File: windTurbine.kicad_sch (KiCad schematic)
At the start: 12 parts, among them M1 Motor_Servo, M2 LP-MSPM0G3507

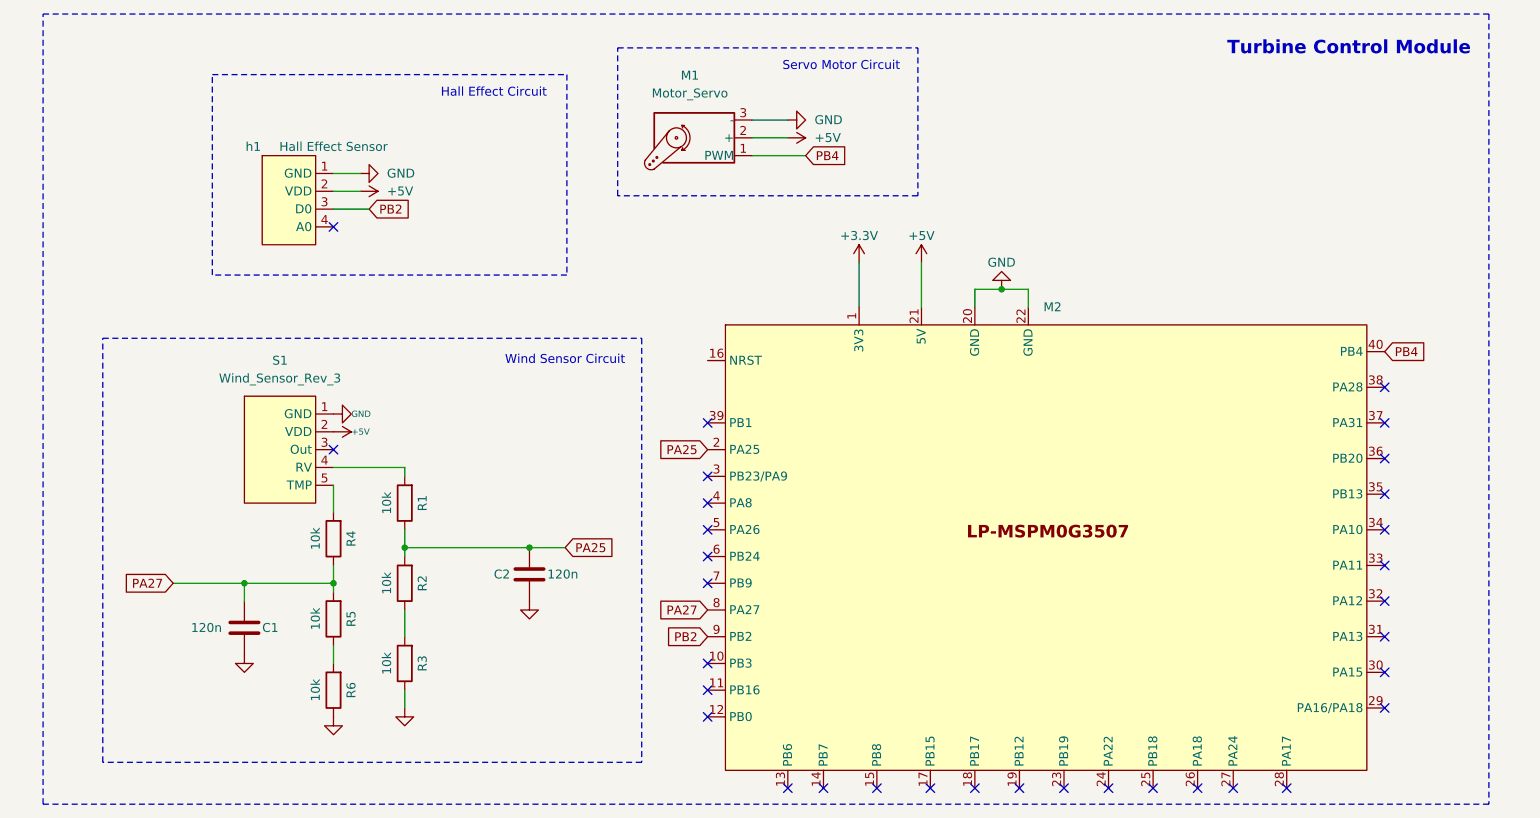
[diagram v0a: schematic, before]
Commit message: Load MCU
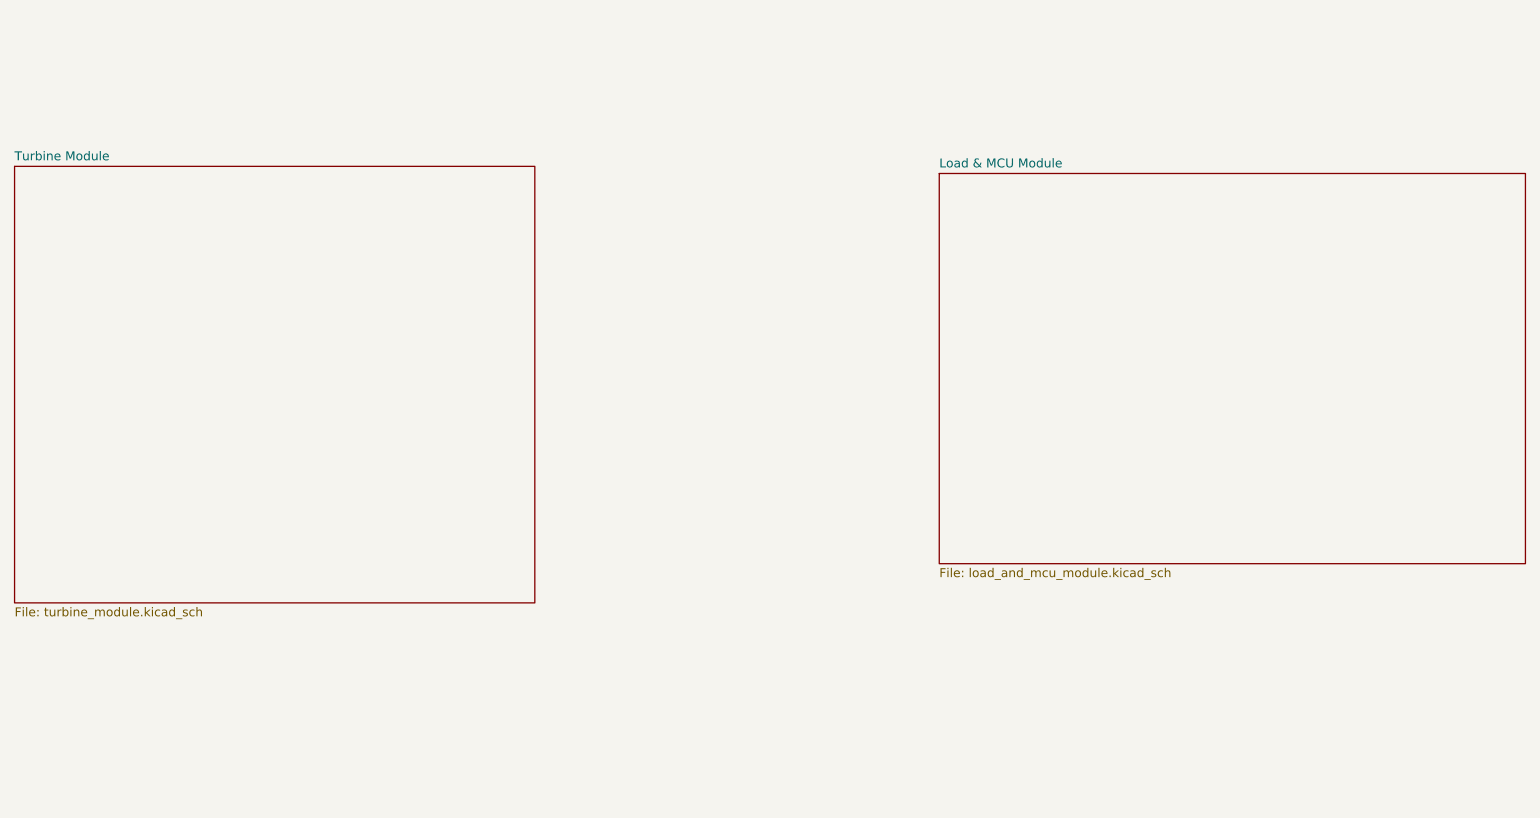
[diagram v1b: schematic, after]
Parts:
- removed C1, C2: 120n, symbol Device:C
- removed M1: Motor_Servo, symbol Motor:Motor_Servo
- removed M2: LP-MSPM0G3507, symbol Turbine_MCU:LP-MSPM0G3507
- removed R1, R2, R3, R4, R5, R6: 10k, symbol Device:R
- removed S1: Wind_Sensor_Rev_3, symbol windTurbineSchemSymLib:Wind_Sensor_Rev_C
- removed h1: Hall Effect Sensor, symbol windTurbineSchemSymLib:hall_effect_sensor
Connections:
- no-connect marks 33 -> 0
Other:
- added sheet Load & MCU Module (load_and_mcu_module.kicad_sch)
- added sheet Turbine Module (turbine_module.kicad_sch)
- note removed: "Hall Effect Circuit"
- note removed: "Servo Motor Circuit"
- note removed: "Turbine Control Module"
- note removed: "Wind Sensor Circuit"
